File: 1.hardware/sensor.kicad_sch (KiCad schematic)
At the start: 0 parts

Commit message: 중간 저장
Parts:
- added AC1: BNO085, BNO085, symbol SamacSys_Parts:BNO085
- added U3: LM75B, symbol Sensor_Temperature:LM75B
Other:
- note added: "IMU"
- note added: "TEMP"

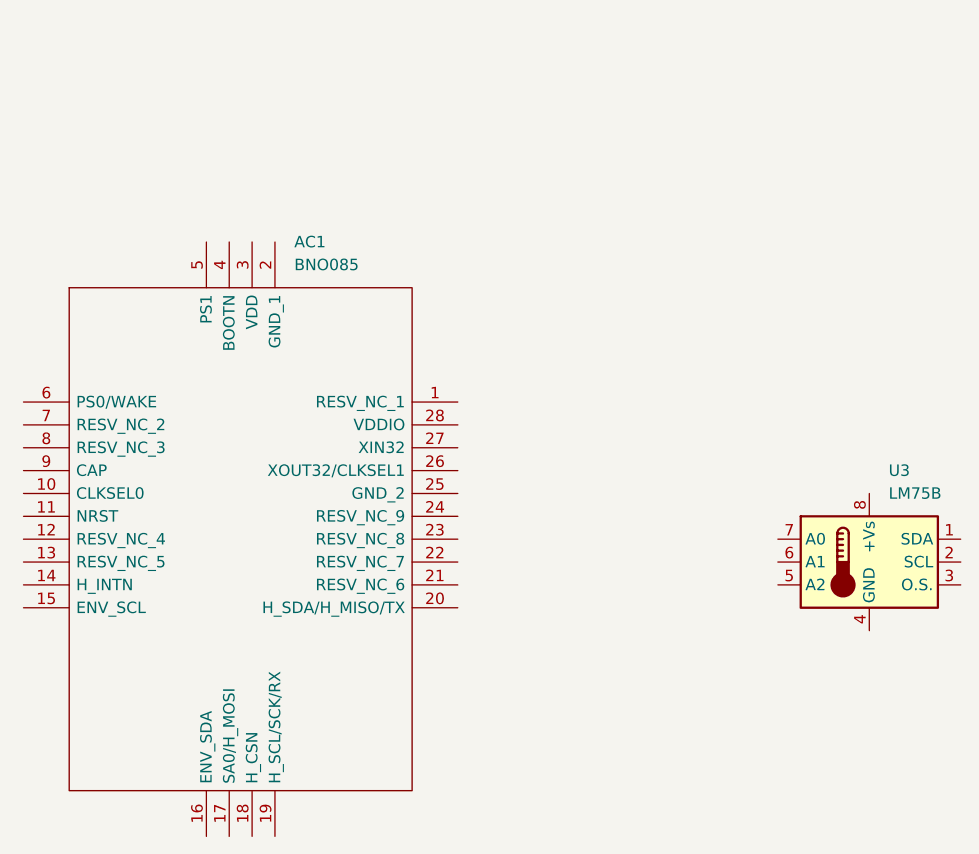
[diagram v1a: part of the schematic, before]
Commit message: 중간 저장2
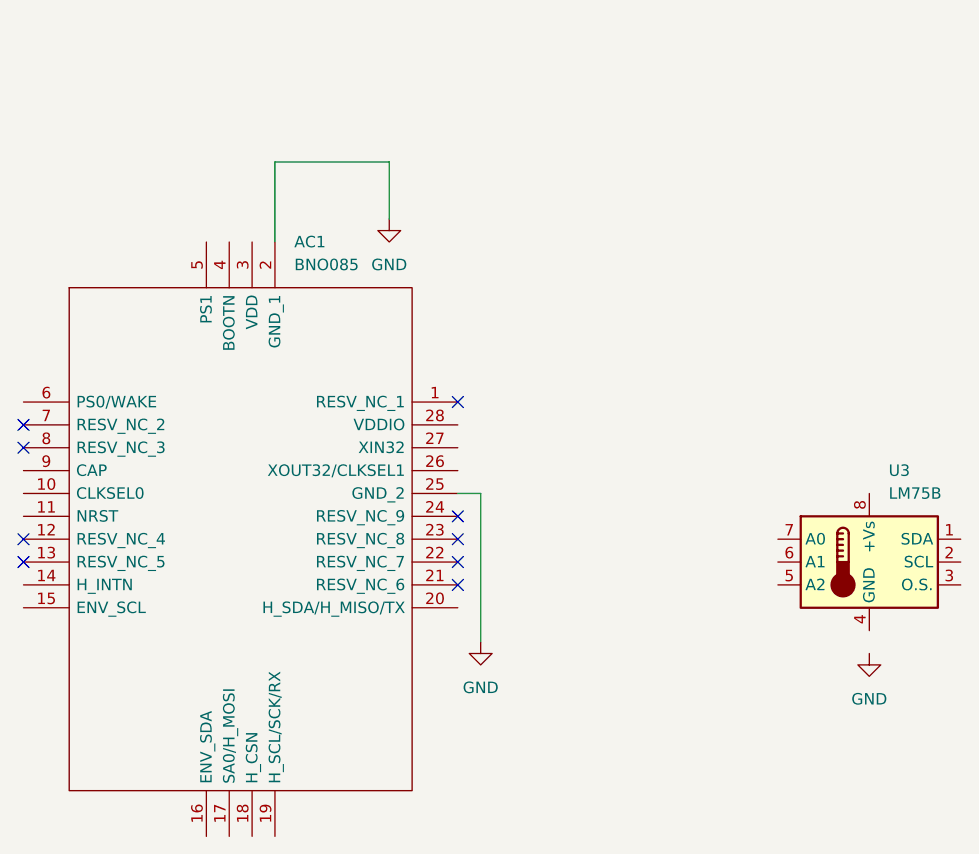
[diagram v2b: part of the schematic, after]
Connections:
- net GND: now reaches AC1.2 (GND_1)
- net GND: now also AC1.25 (GND_2)
- no-connect marks 0 -> 9

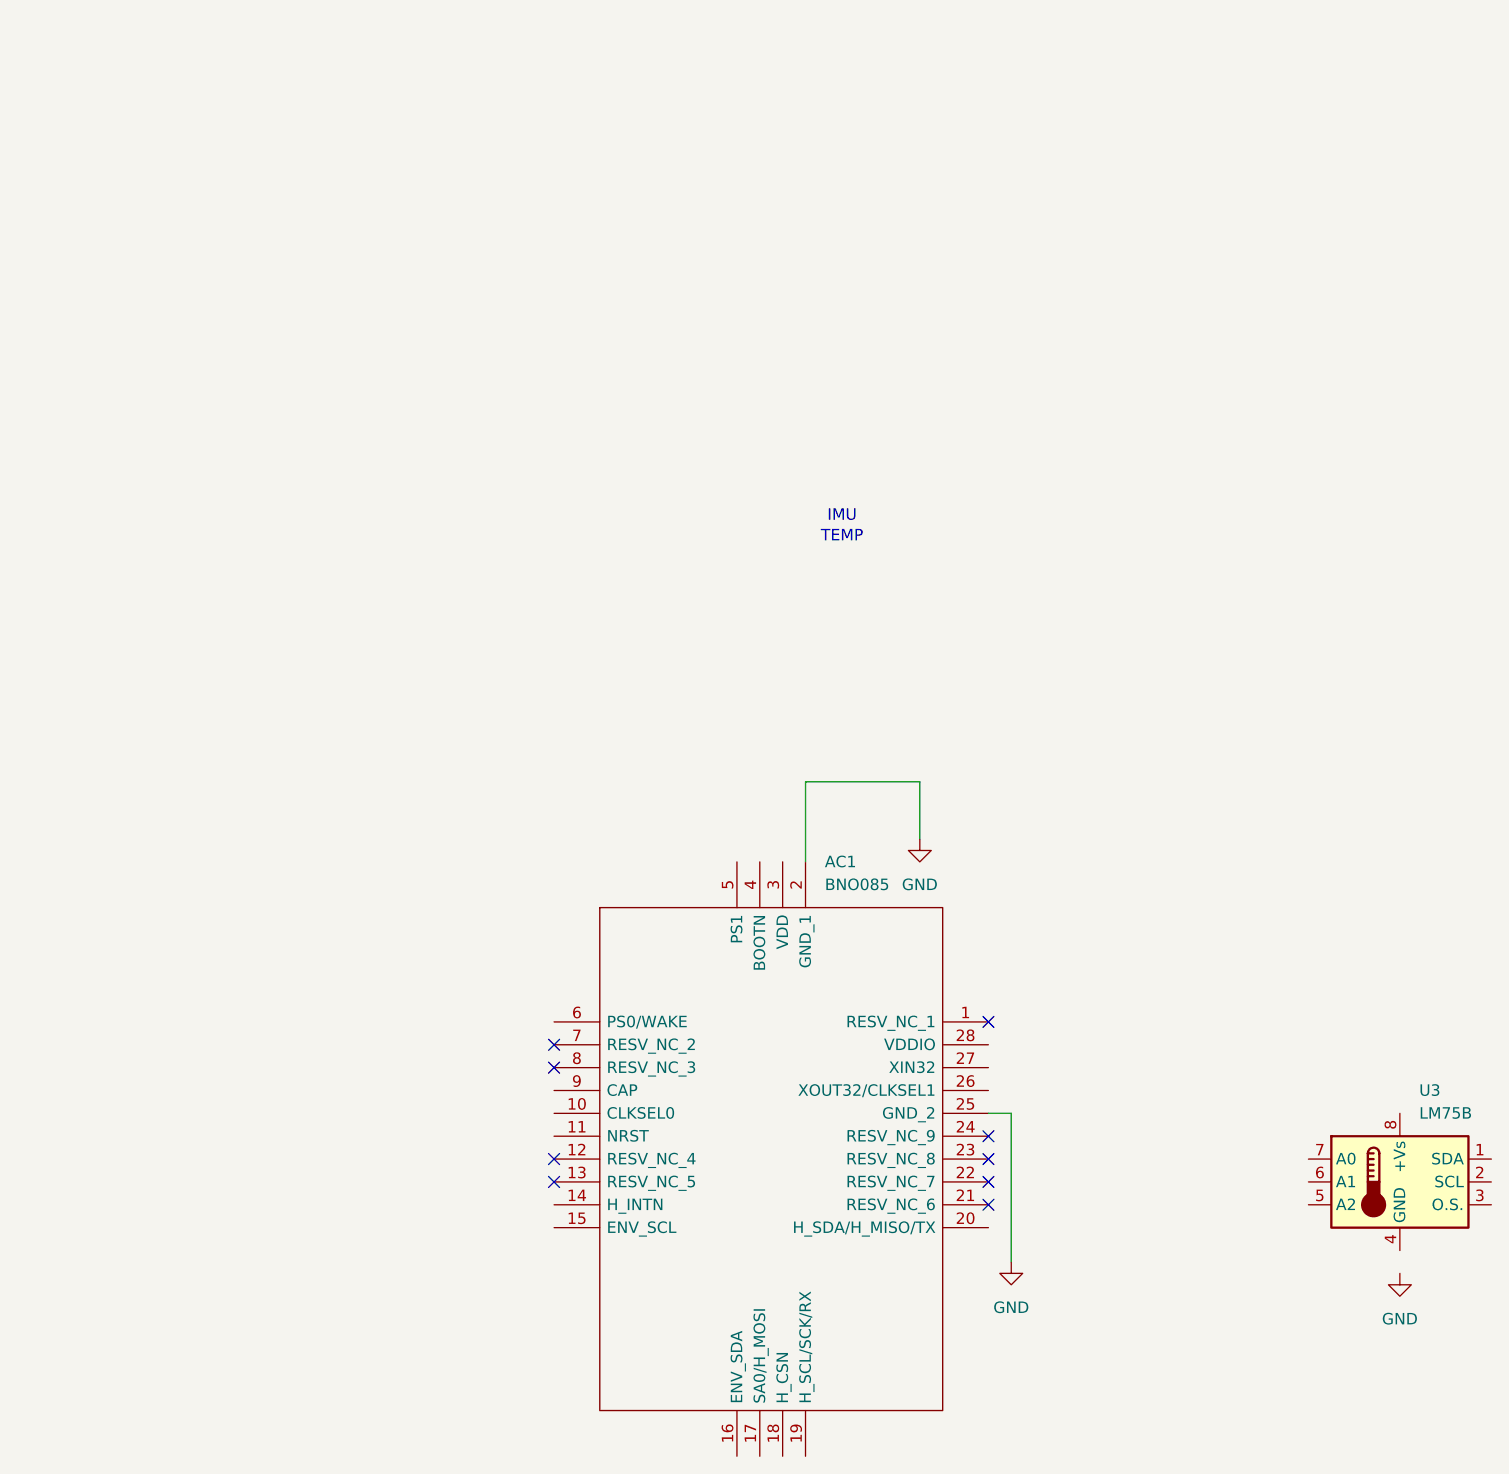
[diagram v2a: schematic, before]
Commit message: 중간 저장
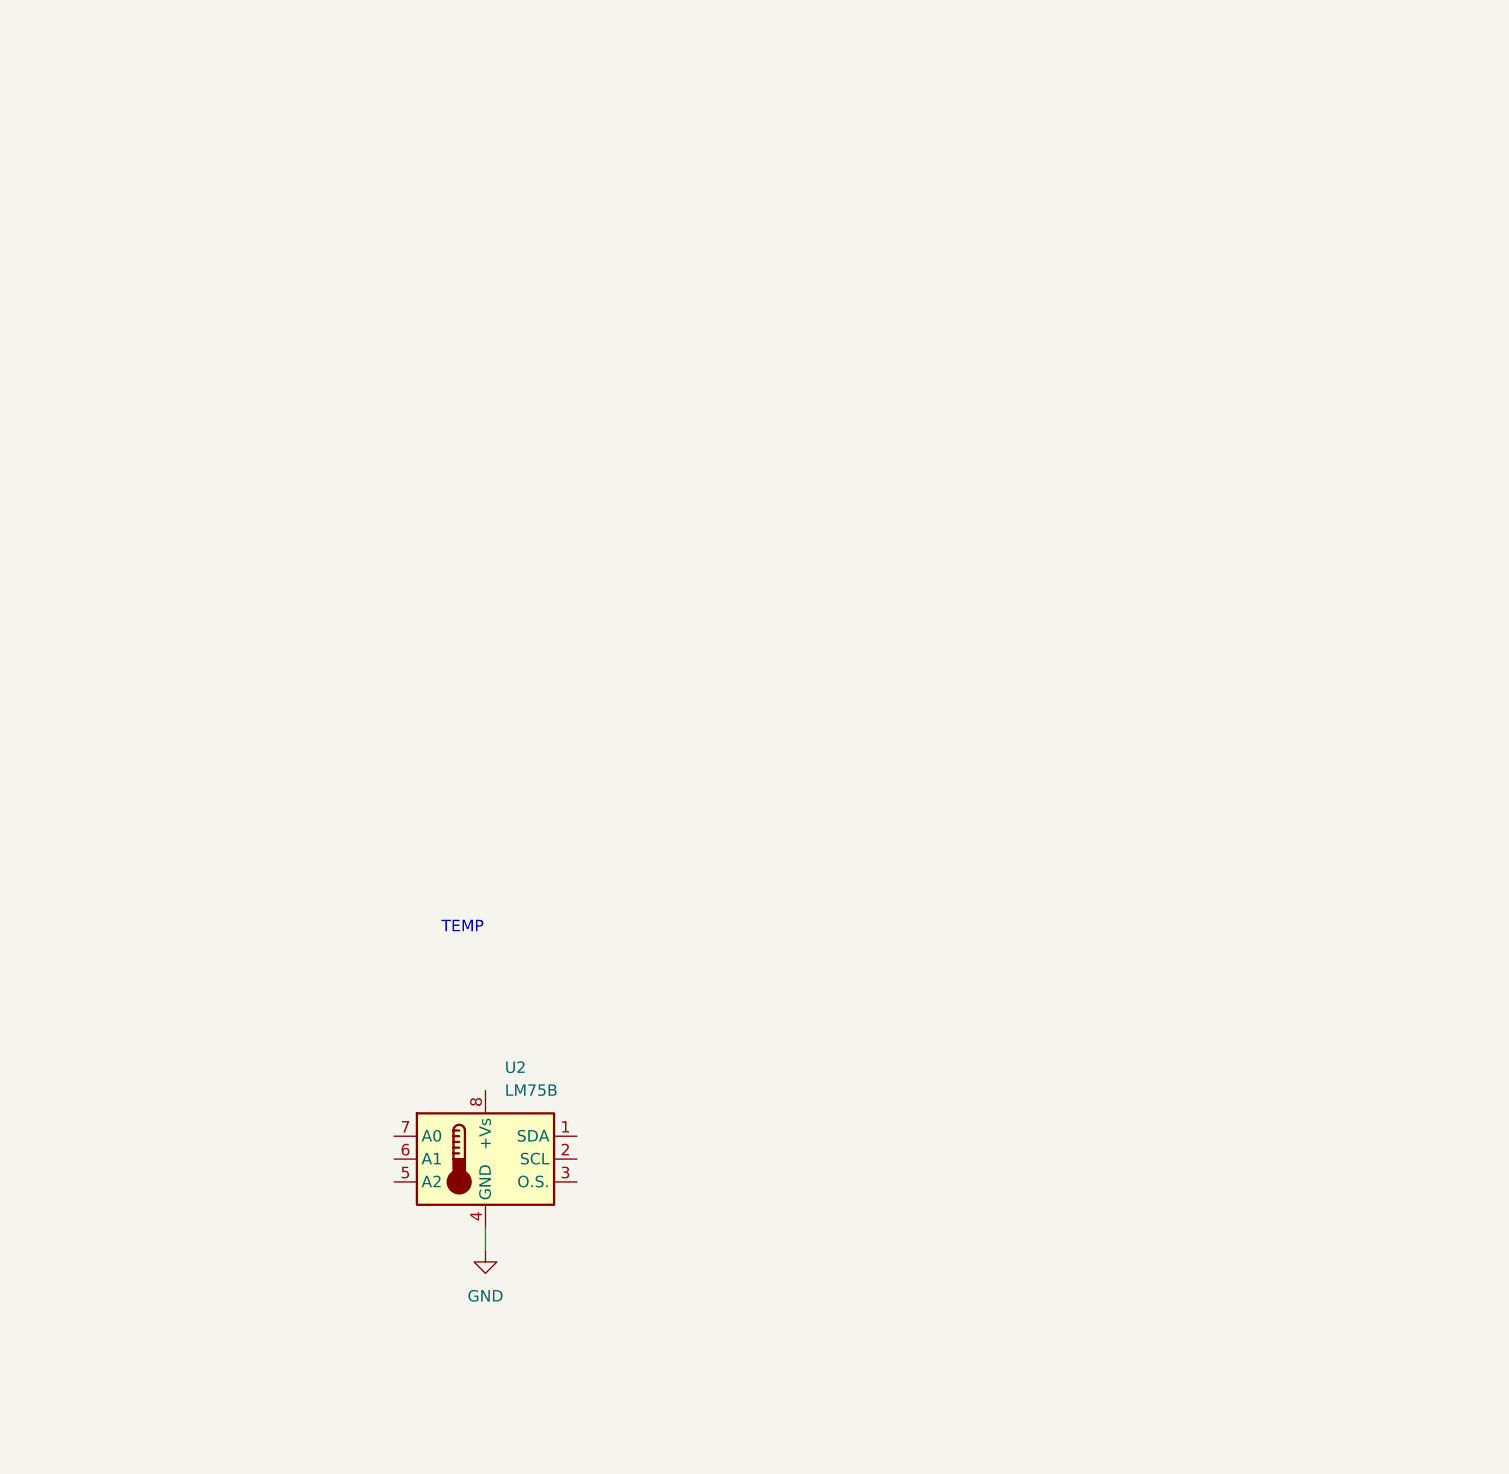
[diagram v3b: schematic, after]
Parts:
- removed AC1: BNO085, BNO085, symbol SamacSys_Parts:BNO085
- renumbered U3 to U2
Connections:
- net GND: now also U2.4 (GND)
- no-connect marks 9 -> 0
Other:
- note removed: "IMU"
- moved on the sheet: U2

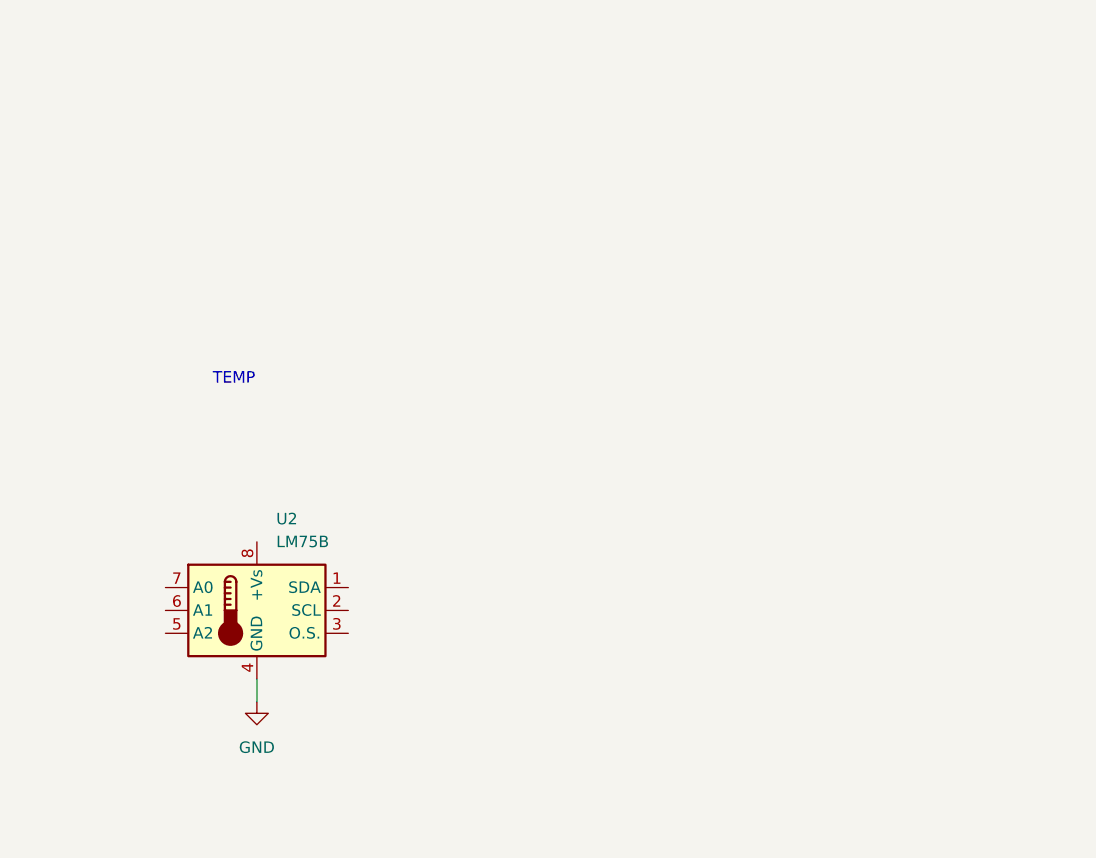
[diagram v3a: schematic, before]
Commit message: 중간 저장
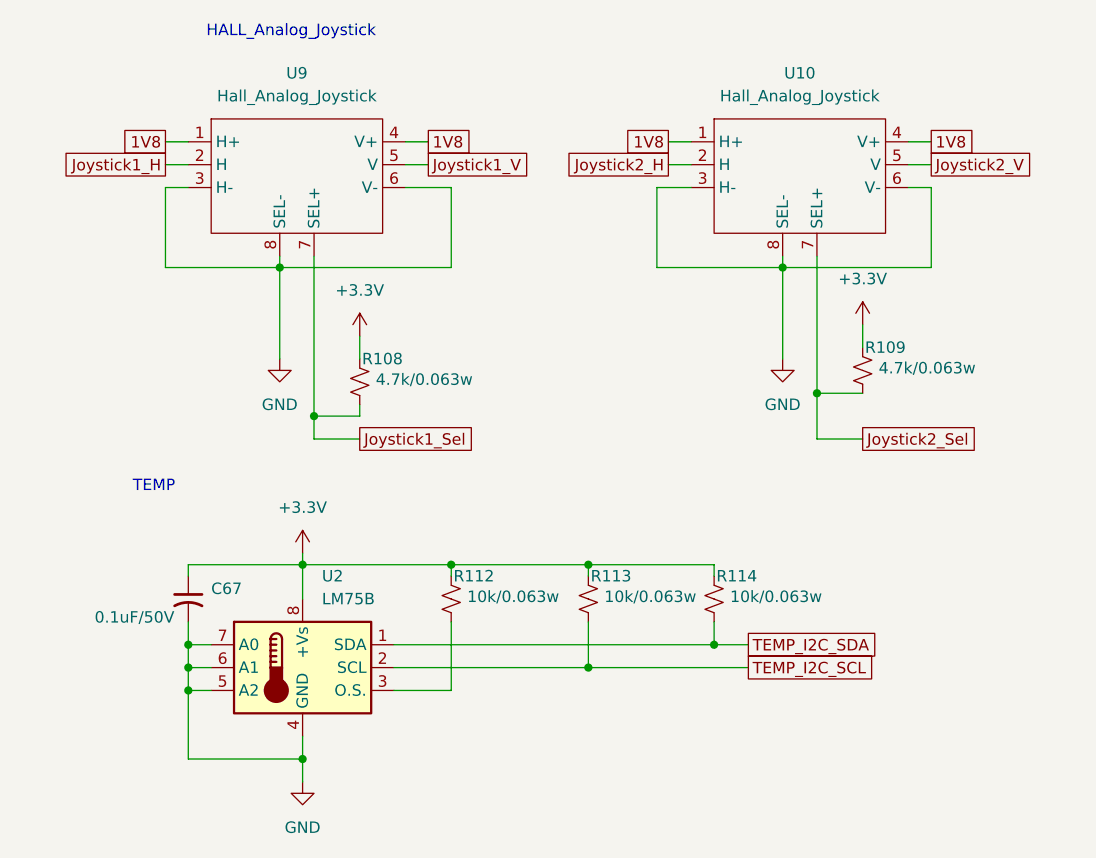
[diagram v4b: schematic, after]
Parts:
- added C67: 0.1uF/50V, Capacitor_SMD:C_0603_1608Metric, symbol Device:C_Small_US
- added R108, R109: 4.7k/0.063w, Resistor_SMD:R_0402_1005Metric, symbol Device:R_Small_US
- added R112, R113, R114: 10k/0.063w, Resistor_SMD:R_0402_1005Metric, symbol Device:R_Small_US
- added U10, U9: Hall_Analog_Joystick, New_Footprints:Hall_Analog_Joystick, symbol New_Library:Hall_Analog_Sensor
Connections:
- net GND: now also U2.5 (A2), U2.6 (A1), U2.7 (A0), C67.2, U10.3 (H-), U10.6 (V-), U10.8 (SEL-), U9.3 (H-), U9.6 (V-), U9.8 (SEL-)
- net TEMP_I2C_SDA: now reaches U2.1 (SDA)
- net TEMP_I2C_SDA: now also R114.2
- net TEMP_I2C_SCL: now reaches U2.2 (SCL)
- net TEMP_I2C_SCL: now also R113.2
- net at U2.3 (O.S.): now also R112.2
- net +3.3V: now reaches U2.8 (+Vs)
- net +3.3V: now also C67.1, R108.1, R109.1, R112.1, R113.1, R114.1
- new net 1V8: U10.1 (H+), U10.4 (V+), U9.1 (H+), U9.4 (V+)
- new net Joystick1_H: U9.2 (H)
- new net Joystick1_Sel: R108.2, U9.7 (SEL+)
- new net Joystick1_V: U9.5 (V)
- new net Joystick2_H: U10.2 (H)
- new net Joystick2_Sel: R109.2, U10.7 (SEL+)
- new net Joystick2_V: U10.5 (V)
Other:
- note added: "HALL_Analog_Joystick"
- moved on the sheet: U2

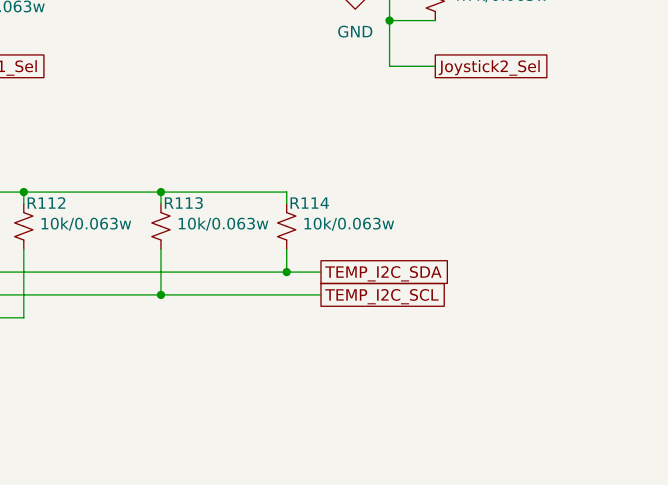
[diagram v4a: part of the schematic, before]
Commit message: 중간 수정
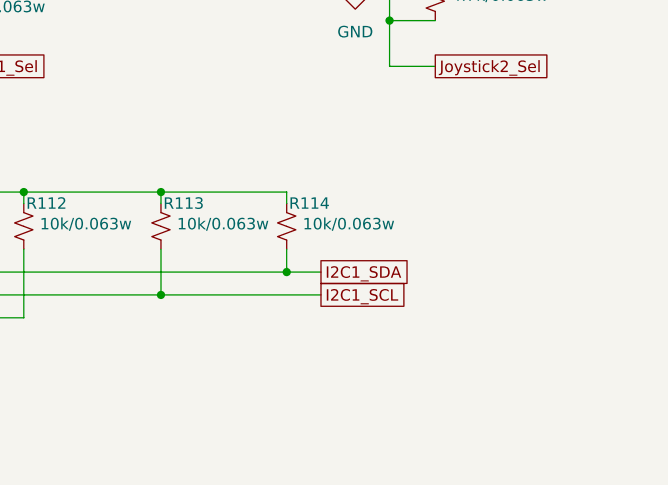
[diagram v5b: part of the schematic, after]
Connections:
- net TEMP_I2C_SCL renamed I2C1_SCL
- net TEMP_I2C_SDA renamed I2C1_SDA
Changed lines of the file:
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@@
 		)
 	)
-	(global_label "TEMP_I2C_SDA"
+	(global_label "I2C1_SDA"
 		(shape passive)
 		(at 132.08 210.82 0)
@@
 		)
 		(property "Intersheetrefs" "${INTERSHEET_REFS}"
-			(at 147.3795 210.82 0)
+			(at 142.7834 210.82 0)
 			(effects
 				(font
@@
 		)
 	)
-	(global_label "TEMP_I2C_SCL"
+	(global_label "I2C1_SCL"
 		(shape passive)
 		(at 132.08 213.36 0)
@@
 		)
 		(property "Intersheetrefs" "${INTERSHEET_REFS}"
-			(at 147.319 213.36 0)
-			(effects
-				(font
+			(at 142.7229 213.36 0)
+			(effects
+				(font
